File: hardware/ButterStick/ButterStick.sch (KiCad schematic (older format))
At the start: 0 parts

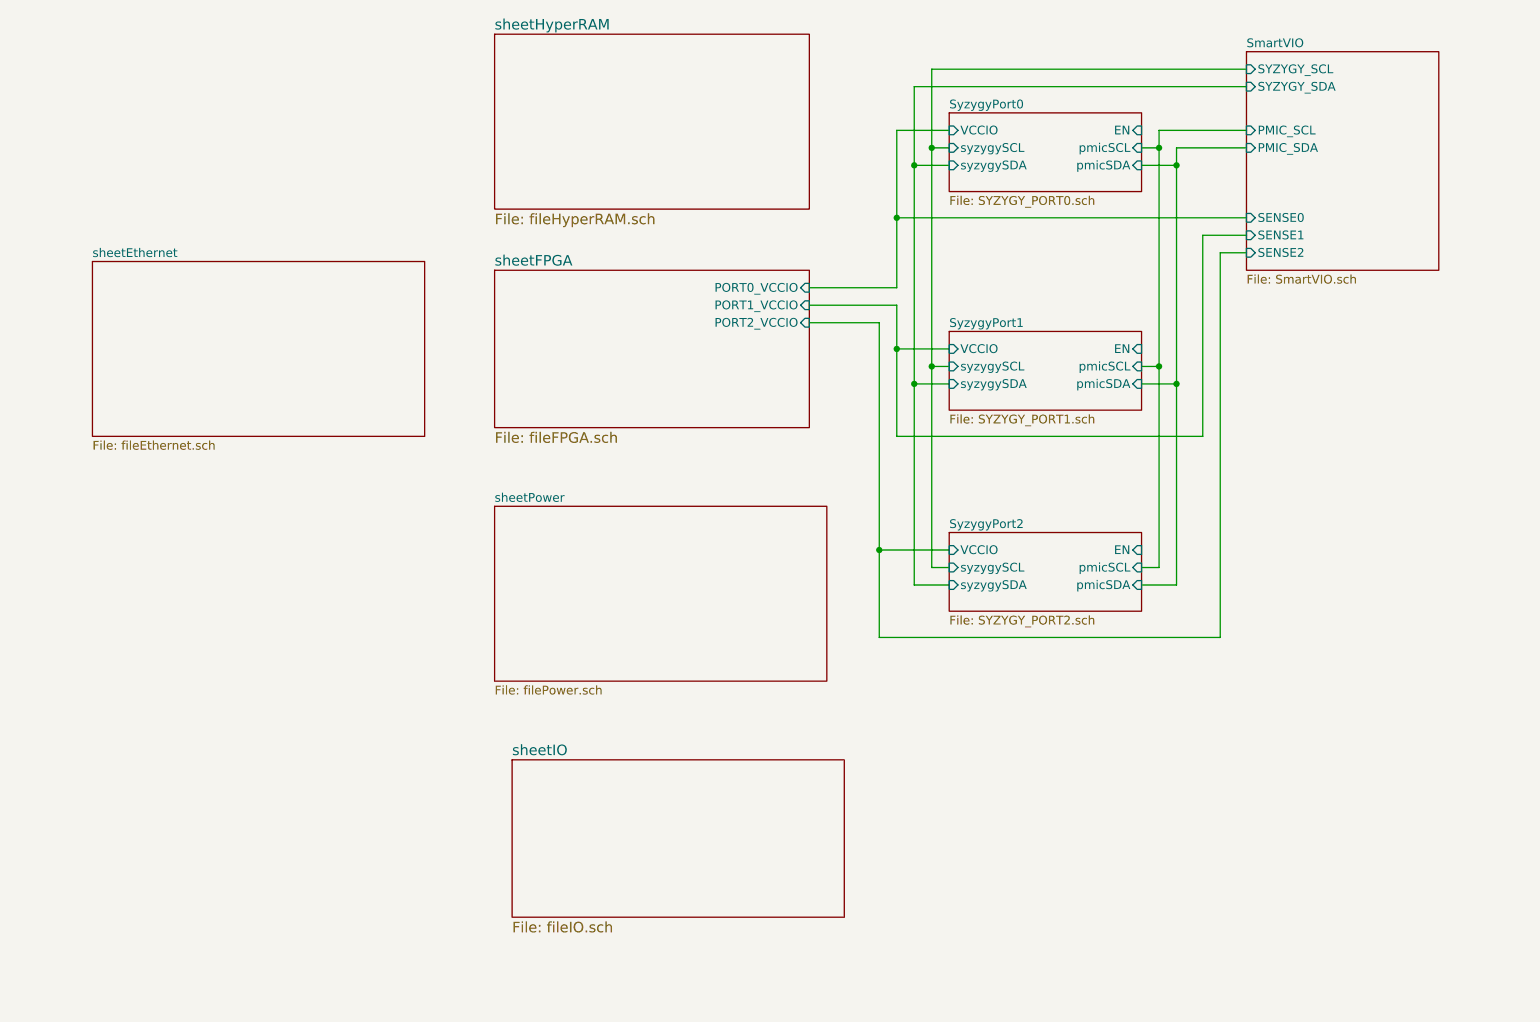
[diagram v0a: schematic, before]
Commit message: Update KiCad PCB.
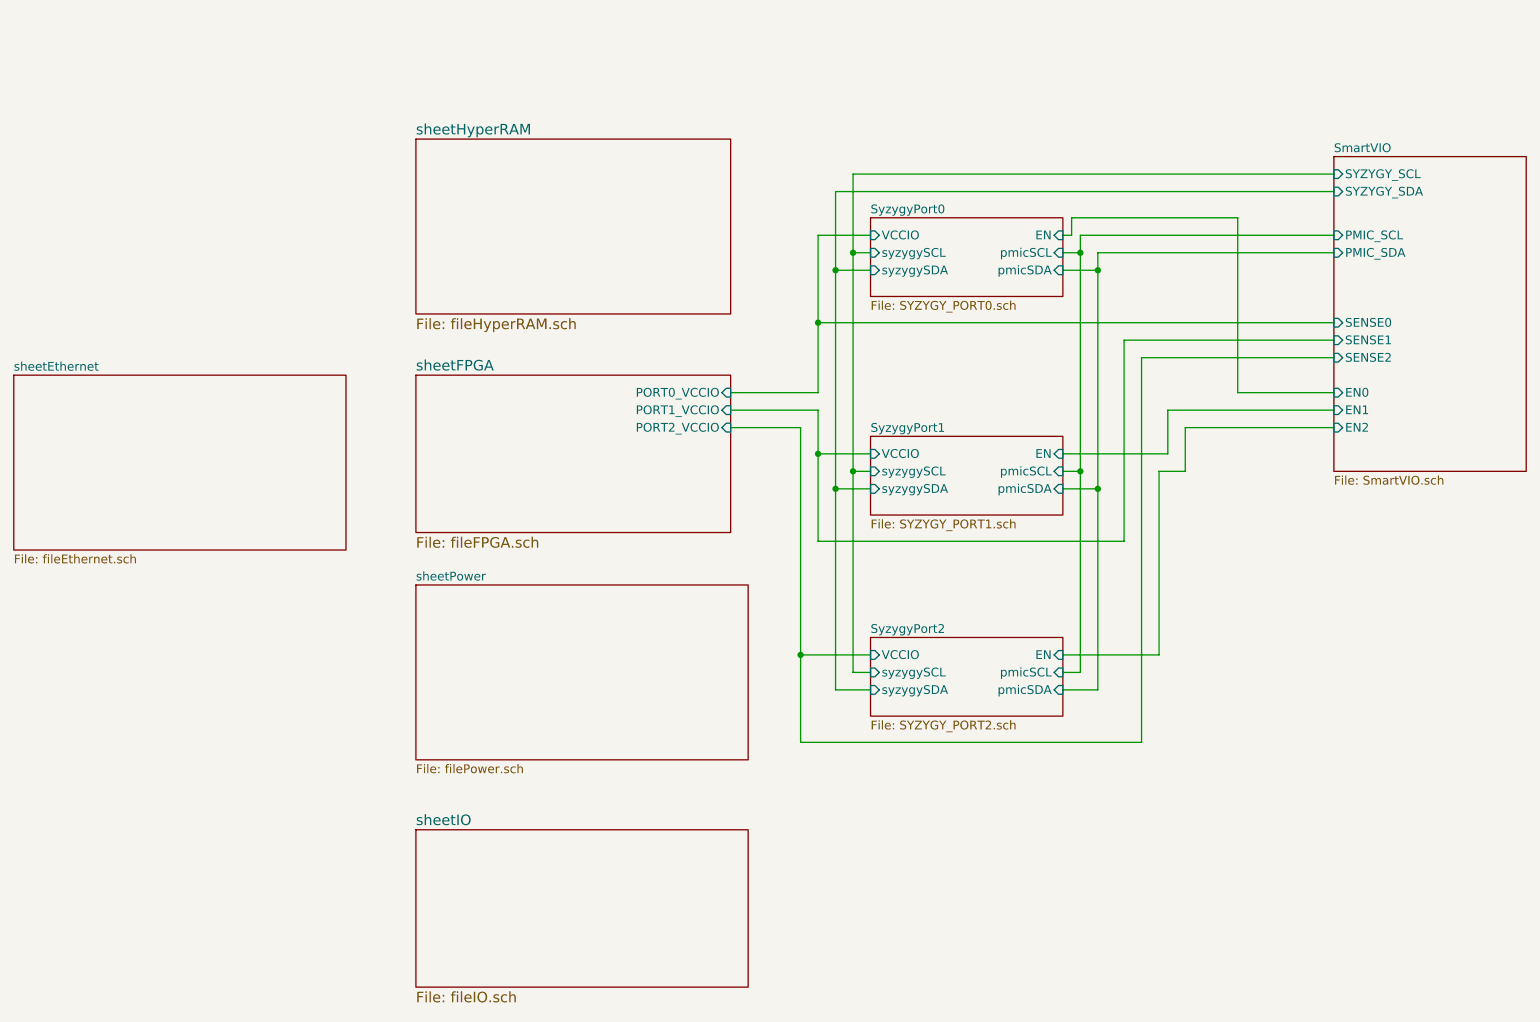
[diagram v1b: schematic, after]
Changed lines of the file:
@@
 $EndDescr
 $Sheet
-S 4600 2450 1800 900
+S 4150 3050 1800 900
 U 5AB8ACB7
 F0 "sheetFPGA" 60
 F1 "fileFPGA.sch" 60
-F2 "PORT0_VCCIO" I R 6400 2550 50
-F3 "PORT1_VCCIO" I R 6400 2650 50
-F4 "PORT2_VCCIO" I R 6400 2750 50
-$EndSheet
-$Sheet
-S 4600 1100 1800 1000
+F2 "PORT0_VCCIO" I R 5950 3150 50
+F3 "PORT1_VCCIO" I R 5950 3250 50
+F4 "PORT2_VCCIO" I R 5950 3350 50
+$EndSheet
+$Sheet
+S 4150 1700 1800 1000
 U 5ABD38F2
 F0 "sheetHyperRAM" 60
@@
 $EndSheet
 $Sheet
-S 4700 5250 1900 900
+S 4150 5650 1900 900
 U 5ABC9A87
 F0 "sheetIO" 60
@@
 $EndSheet
 $Sheet
-S 2300 2400 1900 1000
+S 1850 3050 1900 1000
 U 5BA0BA35
 F0 "sheetEthernet" 50
@@
 $EndSheet
 $Sheet
-S 4600 3800 1900 1000
+S 4150 4250 1900 1000
 U 5BBD18EA
 F0 "sheetPower" 50
@@
 $EndSheet
 $Sheet
-S 7200 1550 1100 450
+S 6750 2150 1100 450
 U 5C80F19A
 F0 "SyzygyPort0" 50
 F1 "SYZYGY_PORT0.sch" 50
-F2 "VCCIO" I L 7200 1650 50
-F3 "syzygySCL" I L 7200 1750 50
-F4 "syzygySDA" I L 7200 1850 50
-F5 "pmicSCL" I R 8300 1750 50
-F6 "pmicSDA" I R 8300 1850 50
-F7 "EN" I R 8300 1650 50
-$EndSheet
-$Sheet
-S 7200 2800 1100 450
+F2 "VCCIO" I L 6750 2250 50
+F3 "syzygySCL" I L 6750 2350 50
+F4 "syzygySDA" I L 6750 2450 50
+F5 "pmicSCL" I R 7850 2350 50
+F6 "pmicSDA" I R 7850 2450 50
+F7 "EN" I R 7850 2250 50
+$EndSheet
+$Sheet
+S 6750 3400 1100 450
 U 5C80F19D
 F0 "SyzygyPort1" 50
 F1 "SYZYGY_PORT1.sch" 50
-F2 "VCCIO" I L 7200 2900 50
-F3 "syzygySCL" I L 7200 3000 50
-F4 "syzygySDA" I L 7200 3100 50
-F5 "pmicSCL" I R 8300 3000 50
-F6 "pmicSDA" I R 8300 3100 50
-F7 "EN" I R 8300 2900 50
-$EndSheet
-$Sheet
-S 7200 3950 1100 450
+F2 "VCCIO" I L 6750 3500 50
+F3 "syzygySCL" I L 6750 3600 50
+F4 "syzygySDA" I L 6750 3700 50
+F5 "pmicSCL" I R 7850 3600 50
+F6 "pmicSDA" I R 7850 3700 50
+F7 "EN" I R 7850 3500 50
+$EndSheet
+$Sheet
+S 6750 4550 1100 450
 U 5C80F1A0
 F0 "SyzygyPort2" 50
 F1 "SYZYGY_PORT2.sch" 50
-F2 "VCCIO" I L 7200 4050 50
-F3 "syzygySCL" I L 7200 4150 50
-F4 "syzygySDA" I L 7200 4250 50
-F5 "pmicSCL" I R 8300 4150 50
-F6 "pmicSDA" I R 8300 4250 50
-F7 "EN" I R 8300 4050 50
-$EndSheet
-Wire Wire Line
-	7200 4150 7100 4150
-Wire Wire Line
-	7100 4150 7100 3000
-Wire Wire Line
-	7100 1750 7200 1750
-Wire Wire Line
-	7200 1850 7000 1850
-Wire Wire Line
-	7000 1850 7000 3100
-Wire Wire Line
-	7000 4250 7200 4250
-Wire Wire Line
-	7200 3100 7000 3100
-Connection ~ 7000 3100
-Wire Wire Line
-	7000 3100 7000 4250
-Wire Wire Line
-	7200 3000 7100 3000
-Connection ~ 7100 3000
-Wire Wire Line
-	7100 3000 7100 1750
-Wire Wire Line
-	7200 1650 6900 1650
-Wire Wire Line
-	6900 1650 6900 2150
-Wire Wire Line
-	6900 2550 6400 2550
-Wire Wire Line
-	7200 2900 6900 2900
-Wire Wire Line
-	6900 2900 6900 2650
-Wire Wire Line
-	6900 2650 6400 2650
-Wire Wire Line
-	7200 4050 6800 4050
-Wire Wire Line
-	6800 4050 6800 2750
-Wire Wire Line
-	6800 2750 6400 2750
-$Sheet
-S 8900 1200 1100 1250
+F2 "VCCIO" I L 6750 4650 50
+F3 "syzygySCL" I L 6750 4750 50
+F4 "syzygySDA" I L 6750 4850 50
+F5 "pmicSCL" I R 7850 4750 50
+F6 "pmicSDA" I R 7850 4850 50
+F7 "EN" I R 7850 4650 50
+$EndSheet
+Wire Wire Line
+	6750 4750 6650 4750
+Wire Wire Line
+	6650 4750 6650 3600
+Wire Wire Line
+	6650 2350 6750 2350
+Wire Wire Line
+	6750 2450 6550 2450
+Wire Wire Line
+	6550 2450 6550 3700
+Wire Wire Line
+	6550 4850 6750 4850
+Wire Wire Line
+	6750 3700 6550 3700
+Connection ~ 6550 3700
+Wire Wire Line
+	6550 3700 6550 4850
+Wire Wire Line
+	6750 3600 6650 3600
+Connection ~ 6650 3600
+Wire Wire Line
+	6650 3600 6650 2350
+Wire Wire Line
+	6750 2250 6450 2250
+Wire Wire Line
+	6450 2250 6450 2750
+Wire Wire Line
+	6450 3150 5950 3150
+Wire Wire Line
+	6750 3500 6450 3500
+Wire Wire Line
+	6450 3500 6450 3250
+Wire Wire Line
+	6450 3250 5950 3250
+Wire Wire Line
+	6750 4650 6350 4650
+Wire Wire Line
+	6350 4650 6350 3350
+Wire Wire Line
+	6350 3350 5950 3350
+$Sheet
+S 9400 1800 1100 1800
 U 5C9D13FE
 F0 "SmartVIO" 50
 F1 "SmartVIO.sch" 50
-F2 "SYZYGY_SDA" I L 8900 1400 50
-F3 "SYZYGY_SCL" I L 8900 1300 50
-F4 "PMIC_SDA" I L 8900 1750 50
-F5 "PMIC_SCL" I L 8900 1650 50
-F6 "SENSE0" I L 8900 2150 50
-F7 "SENSE1" I L 8900 2250 50
-F8 "SENSE2" I L 8900 2350 50
-$EndSheet
-Wire Wire Line
-	6900 2150 8900 2150
-Connection ~ 6900 2150
-Wire Wire Line
-	6900 2150 6900 2550
-Wire Wire Line
-	6900 2900 6900 3400
-Wire Wire Line
-	6900 3400 8650 3400
-Wire Wire Line
-	8650 3400 8650 2250
-Wire Wire Line
-	8650 2250 8900 2250
-Connection ~ 6900 2900
-Wire Wire Line
-	6800 4050 6800 4550
-Wire Wire Line
-	6800 4550 8750 4550
-Wire Wire Line
-	8750 4550 8750 2350
-Wire Wire Line
-	8750 2350 8900 2350
-Connection ~ 6800 4050
-Wire Wire Line
-	8300 4150 8400 4150
-Wire Wire Line
-	8400 4150 8400 3000
-Wire Wire Line
-	8400 1650 8900 1650
-Wire Wire Line
-	8900 1750 8500 1750
-Wire Wire Line
-	8500 1750 8500 1850
-Wire Wire Line
-	8500 4250 8300 4250
-Wire Wire Line
-	8300 3100 8500 3100
-Connection ~ 8500 3100
-Wire Wire Line
-	8500 3100 8500 4250
-Wire Wire Line
-	8300 3000 8400 3000
-Connection ~ 8400 3000
-Wire Wire Line
-	8400 3000 8400 1750
-Wire Wire Line
-	8300 1850 8500 1850
-Connection ~ 8500 1850
-Wire Wire Line
-	8500 1850 8500 3100
-Wire Wire Line
-	8300 1750 8400 1750
-Connection ~ 8400 1750
-Wire Wire Line
-	8400 1750 8400 1650
-Wire Wire Line
-	7000 1850 7000 1400
-Wire Wire Line
-	7000 1400 8900 1400
-Connection ~ 7000 1850
-Wire Wire Line
-	7100 1750 7100 1300
-Wire Wire Line
-	7100 1300 8900 1300
-Connection ~ 7100 1750
+F2 "SYZYGY_SDA" I L 9400 2000 50
+F3 "SYZYGY_SCL" I L 9400 1900 50
+F4 "PMIC_SDA" I L 9400 2350 50
+F5 "PMIC_SCL" I L 9400 2250 50
+F6 "SENSE0" I L 9400 2750 50
+F7 "SENSE1" I L 9400 2850 50
+F8 "SENSE2" I L 9400 2950 50
+F9 "EN0" I L 9400 3150 50
+F10 "EN1" I L 9400 3250 50
+F11 "EN2" I L 9400 3350 50
+$EndSheet
+Wire Wire Line
+	6450 2750 9400 2750
+Connection ~ 6450 2750
+Wire Wire Line
+	6450 2750 6450 3150
+Wire Wire Line
+	6450 3500 6450 4000
+Wire Wire Line
+	6450 4000 8200 4000
+Wire Wire Line
+	8200 4000 8200 2850
+Wire Wire Line
+	8200 2850 9400 2850
+Connection ~ 6450 3500
+Wire Wire Line
+	6350 4650 6350 5150
+Wire Wire Line
+	6350 5150 8300 5150
+Wire Wire Line
+	8300 5150 8300 2950
+Wire Wire Line
+	8300 2950 9400 2950
+Connection ~ 6350 4650
+Wire Wire Line
+	7850 4750 7950 4750
+Wire Wire Line
+	7950 4750 7950 3600
+Wire Wire Line
+	7950 2250 9400 2250
+Wire Wire Line
+	9400 2350 8050 2350
+Wire Wire Line
+	8050 2350 8050 2450
+Wire Wire Line
+	8050 4850 7850 4850
+Wire Wire Line
+	7850 3700 8050 3700
+Connection ~ 8050 3700
+Wire Wire Line
+	8050 3700 8050 4850
+Wire Wire Line
+	7850 3600 7950 3600
+Connection ~ 7950 3600
+Wire Wire Line
+	7950 3600 7950 2350
+Wire Wire Line
+	7850 2450 8050 2450
+Connection ~ 8050 2450
+Wire Wire Line
+	8050 2450 8050 3700
+Wire Wire Line
+	7850 2350 7950 2350
+Connection ~ 7950 2350
+Wire Wire Line
+	7950 2350 7950 2250
+Wire Wire Line
+	6550 2450 6550 2000
+Wire Wire Line
+	6550 2000 9400 2000
+Connection ~ 6550 2450
+Wire Wire Line
+	6650 2350 6650 1900
+Wire Wire Line
+	6650 1900 9400 1900
+Connection ~ 6650 2350
+Wire Wire Line
+	7850 2250 7900 2250
+Wire Wire Line
+	7900 2250 7900 2150
+Wire Wire Line
+	7900 2150 8850 2150
+Wire Wire Line
+	8850 2150 8850 3150
+Wire Wire Line
+	8850 3150 9400 3150
+Wire Wire Line
+	9400 3250 8450 3250
+Wire Wire Line
+	8450 3250 8450 3500
+Wire Wire Line
+	8450 3500 7850 3500
+Wire Wire Line
+	7850 4650 8400 4650
+Wire Wire Line
+	8400 4650 8400 3600
+Wire Wire Line
+	8400 3600 8550 3600
+Wire Wire Line
+	8550 3600 8550 3350
+Wire Wire Line
+	8550 3350 9400 3350
 $EndSCHEMATC
